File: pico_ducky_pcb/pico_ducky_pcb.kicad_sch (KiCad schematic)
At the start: 31 parts, among them J1 USB_A, J2 Conn_01x03_Female, SW1 R-667799, SW2 R-667799, U1 AP2138N-3.3, U2 W25Q32JVZP, U3 RP2040, Y1 Crystal_GND24

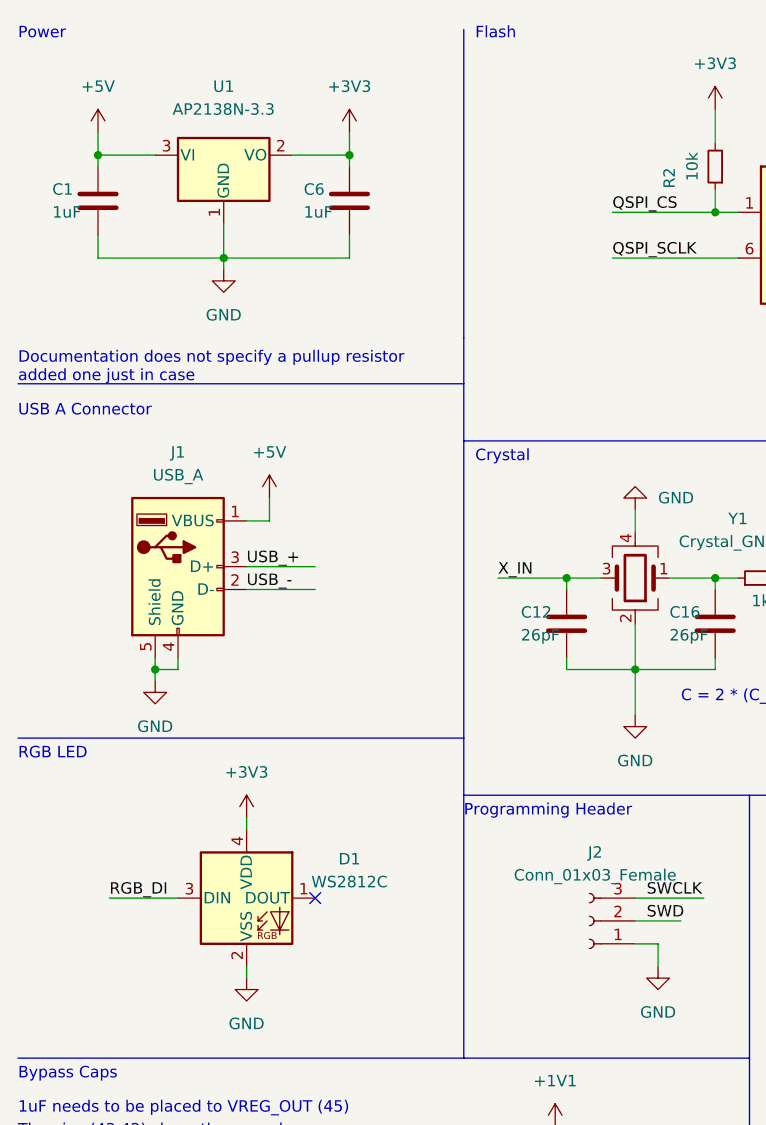
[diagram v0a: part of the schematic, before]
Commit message: pass erc
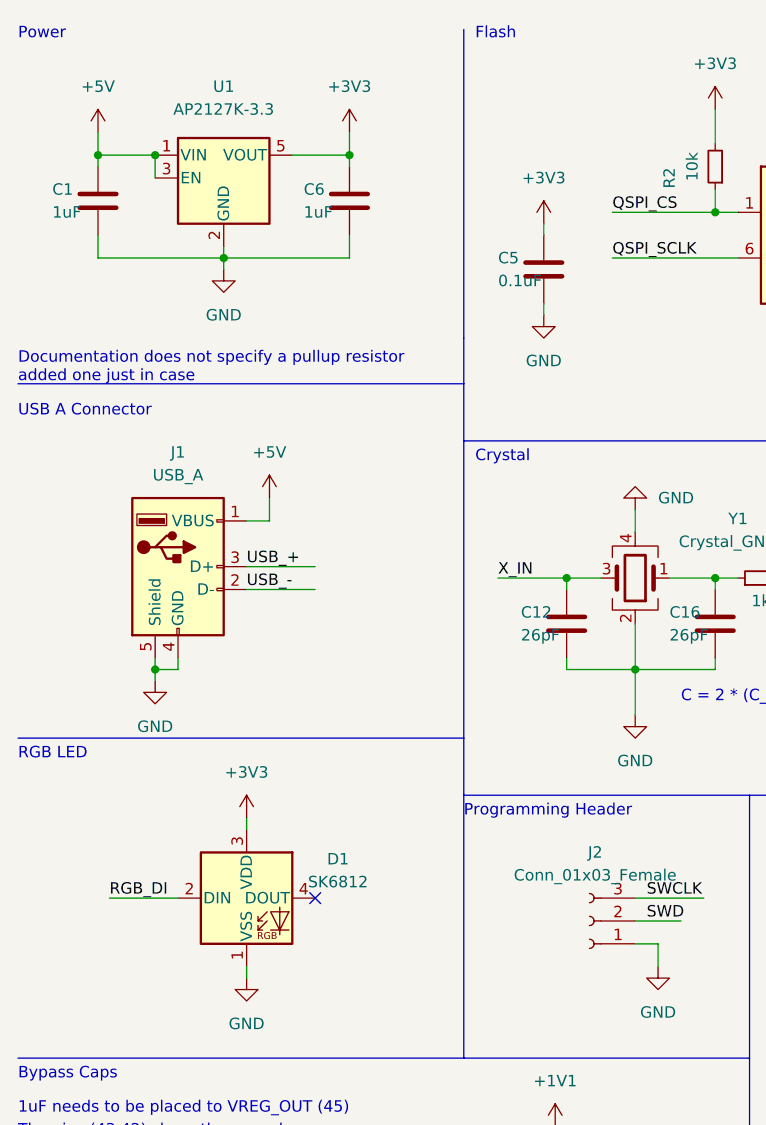
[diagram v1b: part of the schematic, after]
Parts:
- removed D1: WS2812C, WS2812C:WS2812C-2020, symbol LED:WS2812C
- removed U1: AP2138N-3.3, Package_TO_SOT_SMD:SOT-23, symbol Regulator_Linear:AP2138N-3.3
- added C5: 0.1uF, Capacitor_SMD:C_0201_0603Metric, symbol Device:C
- added D1: SK6812, LED_SMD:LED_SK6812_EC15_1.5x1.5mm, symbol LED:SK6812
- added U1: AP2127K-3.3, Package_TO_SOT_SMD:SOT-23-5, symbol Regulator_Linear:AP2127K-3.3
- C10, C11, C13, C15, C3, C4, C7, C8, C9: footprint Capacitor_SMD:C_0402_1005Metric -> Capacitor_SMD:C_0201_0603Metric
- R6, R7: footprint Resistor_SMD:R_0201_0603Metric -> Resistor_SMD:R_0402_1005Metric
- SW1: footprint R-WHATEVER:R-667799 -> (none)
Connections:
- net +3V3: now also C5.2, D1.3 (VDD), U1.5 (VOUT)
- net +5V: now also U1.1 (VIN), U1.3 (EN)
- net GND: now also C5.1, D1.1 (VSS), U1.2 (GND)
- net RGB_DI: now also D1.2 (DIN)
